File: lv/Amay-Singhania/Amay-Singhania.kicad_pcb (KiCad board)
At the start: 4 copper layers, 177.4 x 195.2 mm, 26 parts, among them U1 ADS127L01xPBS, U2 AD8222HACPZ-R7

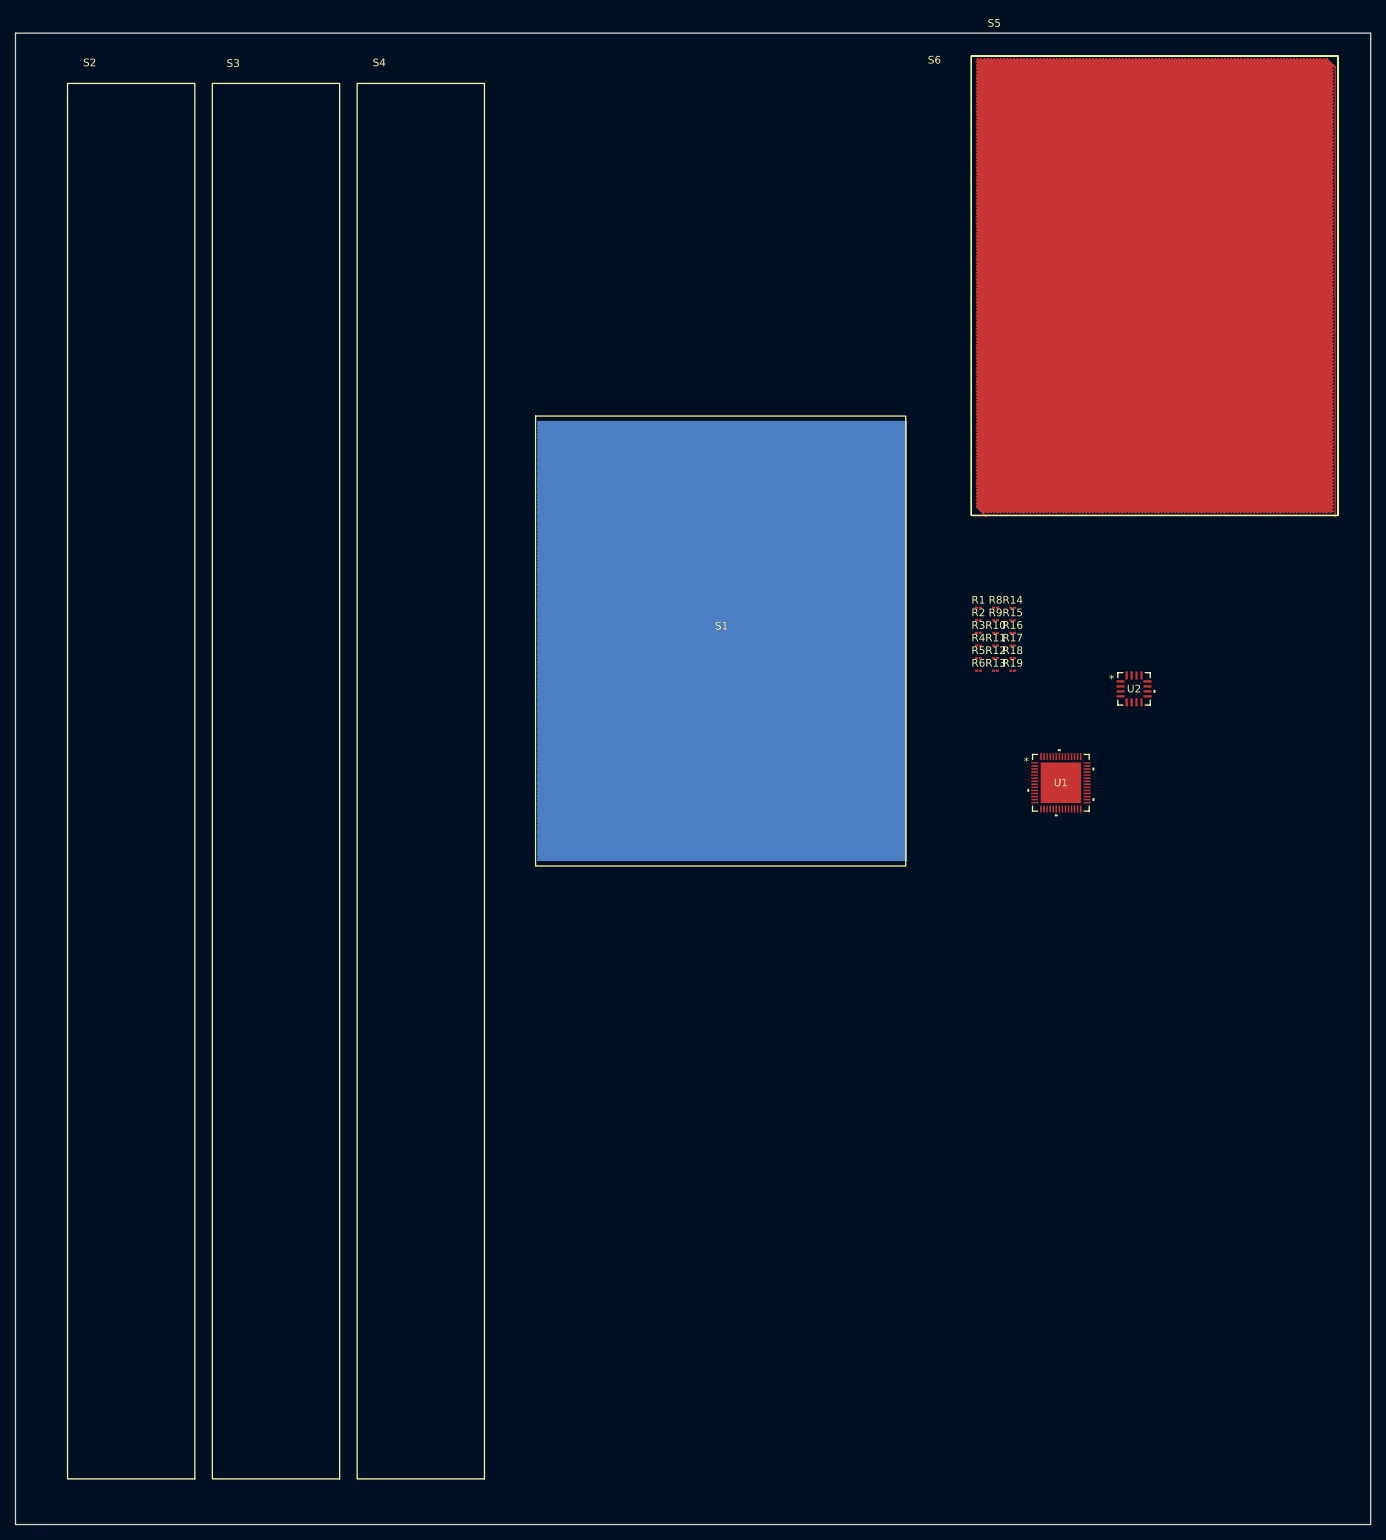
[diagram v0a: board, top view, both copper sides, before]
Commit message: lv and fw changes
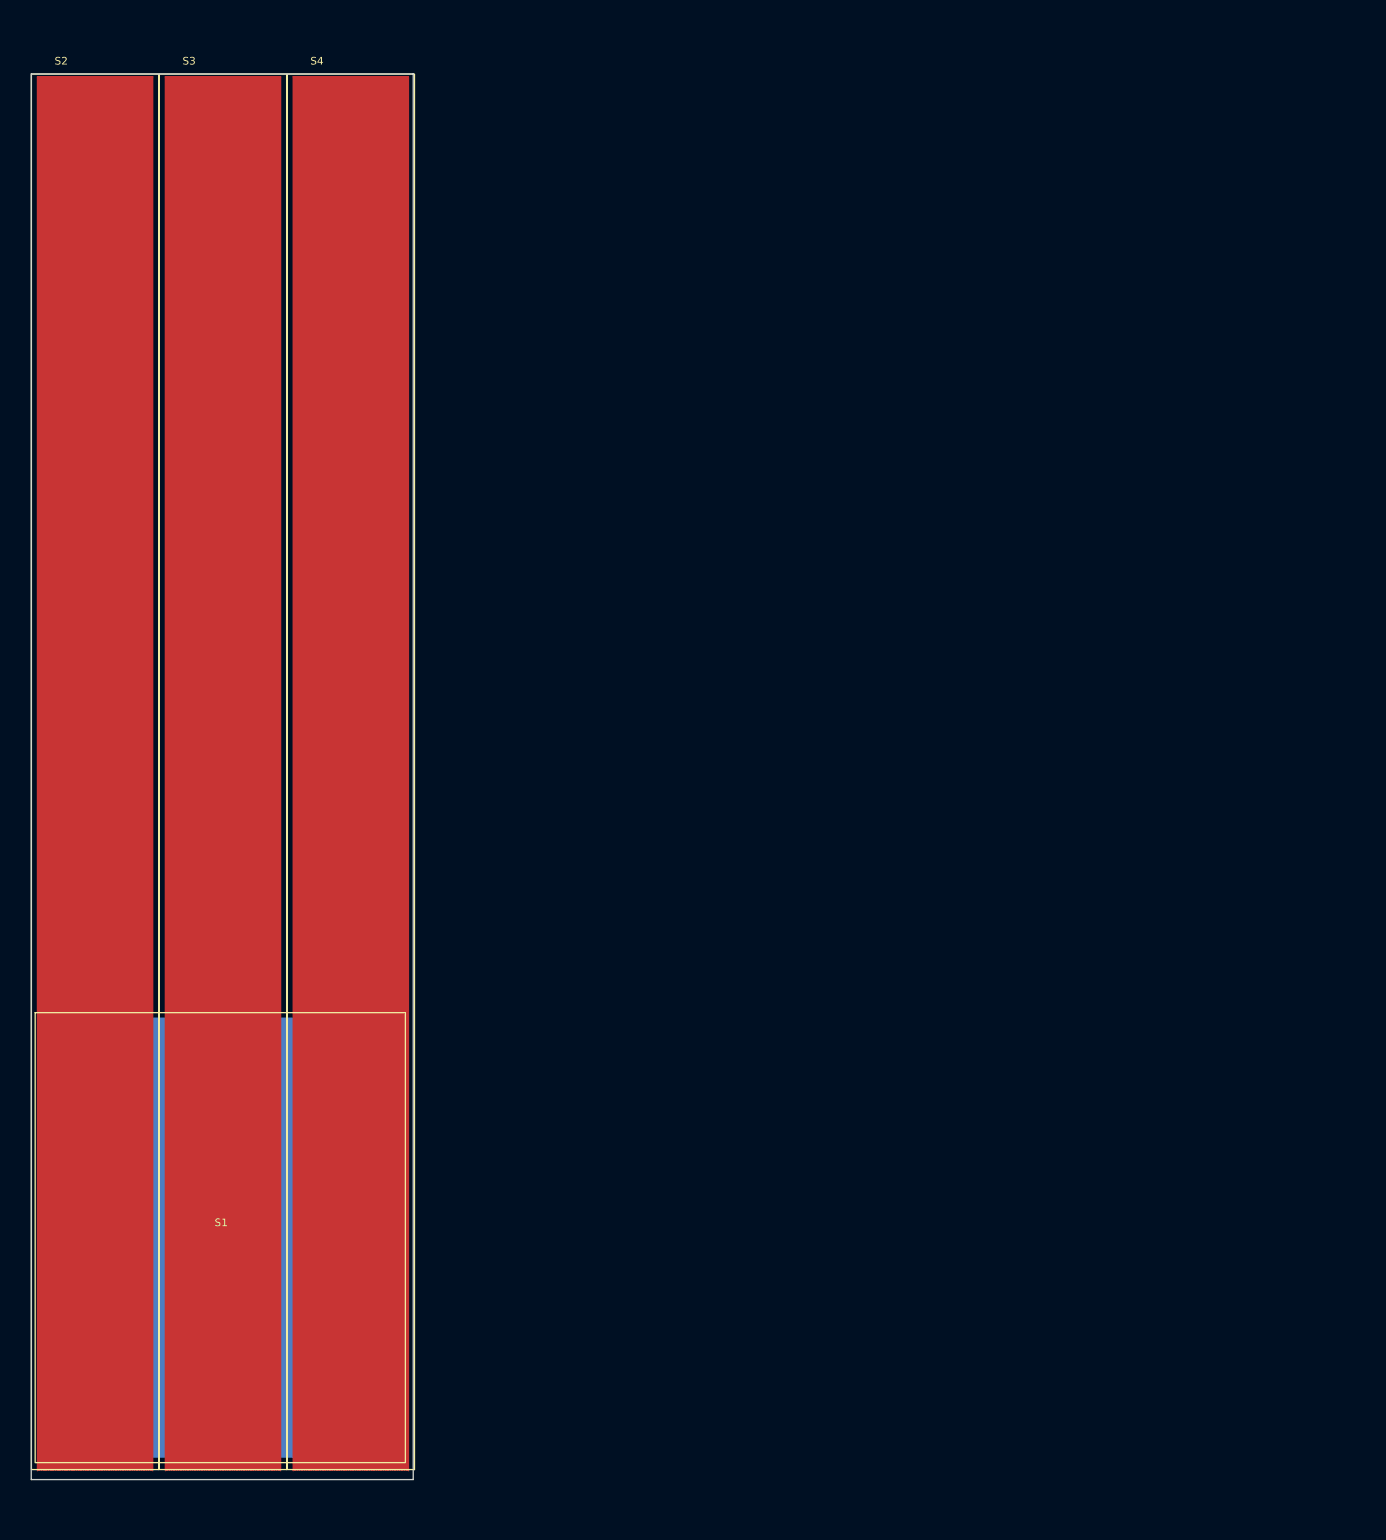
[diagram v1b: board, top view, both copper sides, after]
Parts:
- removed R1, R10, R11, R12, R13, R14, R15, R16, R17, R18, R19, R2, R3, R4, R5, R6, R8, R9: 350, Resistor_SMD:R_01005_0402Metric
- removed S5: StrainGauge, StrainGauge:TorsionalGauge-45deg
- removed S6: StrainGauge, StrainGauge:TorsionalGauge45deg
- removed U1: ADS127L01xPBS, ADS127L01xPBS:VQFN56_RSH_TEX
- removed U2: AD8222HACPZ-R7, AD8222:CP_16_19_ADI
- S2, S3, S4: value StrainGauge -> StrainGaugeAxial
- moved S1 101.9 mm to (41.9, 167.9)
- moved S4 8.16 mm to (50.5, 17.0)
- moved S3 5.94 mm to (33.8, 17.0)
- moved S2 3.73 mm to (17.0, 17.0)
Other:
- board size 177.4 x 195.2 mm -> 50 x 184 mm
